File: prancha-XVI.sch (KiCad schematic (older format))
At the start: 11 parts

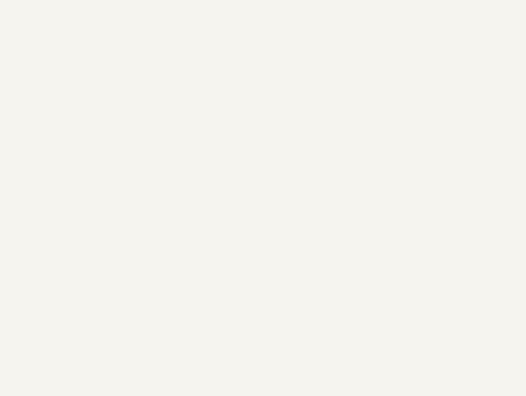
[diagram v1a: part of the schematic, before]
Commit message: mais um pedação do esquemático (prancha XIV)
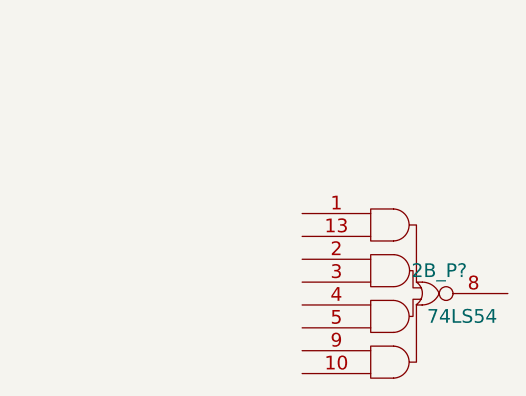
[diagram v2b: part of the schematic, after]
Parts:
- added 2B_P?: 74LS54, ~, symbol 74LS54
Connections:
- net GND: now also 2B_P?.7 (GND)
- net VCC: now also 2B_P?.14 (VCC)
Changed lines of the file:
@@
 LIBS:valves
 LIBS:7451
+LIBS:7454
+LIBS:7460
 LIBS:patinhofeio-cache
 EELAYER 25 0
@@
 Text Notes 12450 6250 0    60   ~ 0
 "Vai Um Quente"
+$Comp
+L 74LS54 2B_P?
+U 1 1 586D7CA5
+P 46050 18300
+F 0 "2B_P?" H 46200 18400 60  0000 C CNN
+F 1 "74LS54" H 46300 18200 60  0000 C CNN
+F 2 "~" H 46050 18300 60  0000 C CNN
+F 3 "~" H 46050 18300 60  0000 C CNN
+	1    46050 18300
+	1    0    0    -1
+$EndComp
 $EndSCHEMATC

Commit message: mais um pouco...
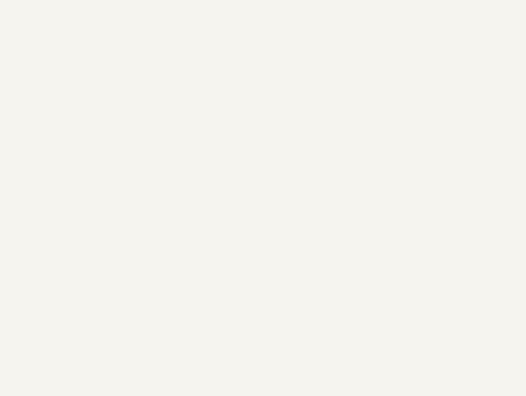
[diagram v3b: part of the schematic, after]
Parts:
- removed 2B_P?: 74LS54, ~, symbol 74LS54
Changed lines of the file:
@@
 Text Notes 12450 6250 0    60   ~ 0
 "Vai Um Quente"
-$Comp
-L 74LS54 2B_P?
-U 1 1 586D7CA5
-P 46050 18300
-F 0 "2B_P?" H 46200 18400 60  0000 C CNN
-F 1 "74LS54" H 46300 18200 60  0000 C CNN
-F 2 "~" H 46050 18300 60  0000 C CNN
-F 3 "~" H 46050 18300 60  0000 C CNN
-	1    46050 18300
-	1    0    0    -1
-$EndComp
 $EndSCHEMATC
